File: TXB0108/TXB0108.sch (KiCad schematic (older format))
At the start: 6 parts, among them J1 Conn_01x10, J2 Conn_01x10, U1 TXB0108DQSR

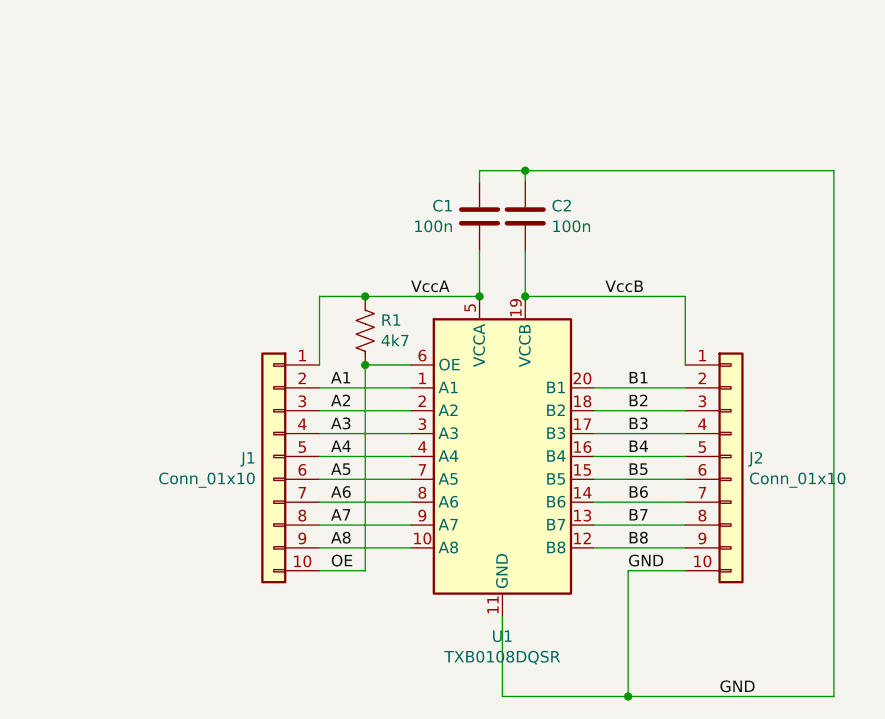
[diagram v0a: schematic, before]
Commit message: Part Numbers Added
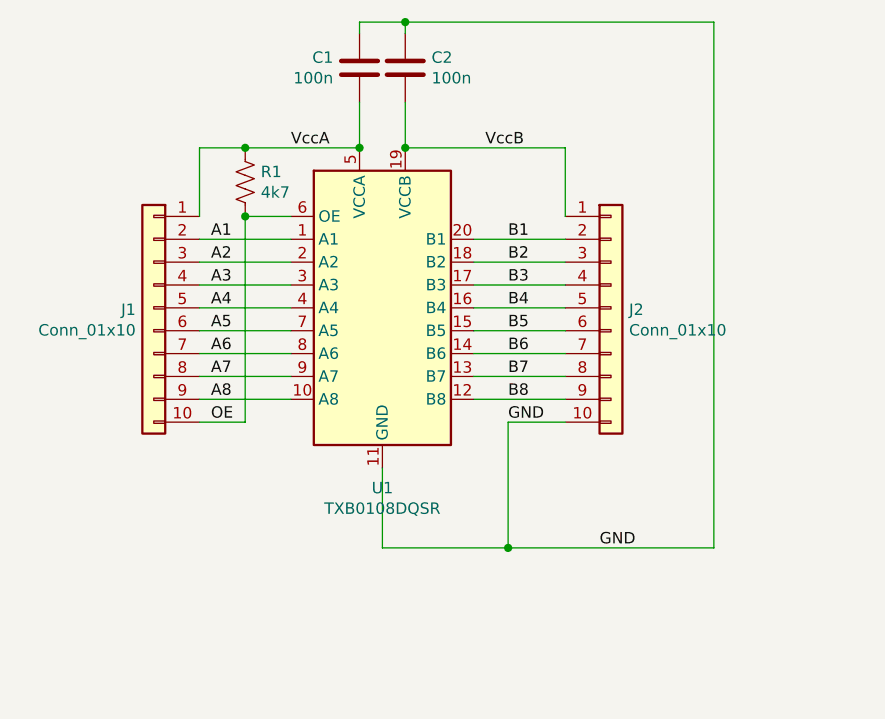
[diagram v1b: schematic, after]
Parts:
- C1, C2: Part (none) -> C38141
- R1: Part (none) -> C99782
- U1: Part (none) -> C53406
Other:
- moved on the sheet: C1, C2, J1, J2, R1, U1
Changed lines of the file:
@@
 EESchema Schematic File Version 4
+LIBS:TXB0108-cache
 EELAYER 29 0
 EELAYER END
-$Descr A4 11693 8268
+$Descr User 8268 5807
 encoding utf-8
 Sheet 1 1
-Title ""
-Date ""
-Rev ""
-Comp ""
-Comment1 ""
-Comment2 ""
-Comment3 ""
+Title "8 Channel Bi-Directional Level Shifter"
+Date "2019-09-16"
+Rev "1"
+Comp "SirBoard"
+Comment1 "www.SirBoard.com"
+Comment2 "TXB0108"
+Comment3 "SirLevel"
 Comment4 ""
 $EndDescr
@@
 L Logic_LevelTranslator:TXB0108DQSR U1
 U 1 1 5D2EEB39
-P 4250 3150
-F 0 "U1" H 4250 2362 50  0000 C CNN
-F 1 "TXB0108DQSR" H 4250 2272 50  0000 C CNN
-F 2 "Package_SO:TSSOP-20_4.4x6.5mm_P0.65mm" H 4250 2400 50  0001 C CNN
-F 3 "http://www.ti.com/lit/ds/symlink/txb0108.pdf" H 4250 3050 50  0001 C CNN
-	1    4250 3150
+P 3725 2500
+F 0 "U1" H 3725 1712 50  0000 C CNN
+F 1 "TXB0108DQSR" H 3725 1622 50  0000 C CNN
+F 2 "Package_SO:TSSOP-20_4.4x6.5mm_P0.65mm" H 3725 1750 50  0001 C CNN
+F 3 "http://www.ti.com/lit/ds/symlink/txb0108.pdf" H 3725 2400 50  0001 C CNN
+F 4 "C53406" H 3725 2500 50  0001 C CNN "Part"
+	1    3725 2500
 	1    0    0    -1
 $EndComp
@@
 L Connector_Generic:Conn_01x10 J2
 U 1 1 5D2EF020
-P 5250 3150
-F 0 "J2" H 5329 3142 50  0000 L CNN
-F 1 "Conn_01x10" H 5329 3052 50  0000 L CNN
-F 2 "Connector_PinHeader_2.54mm:PinHeader_1x10_P2.54mm_Vertical" H 5250 3150 50  0001 C CNN
-F 3 "~" H 5250 3150 50  0001 C CNN
-	1    5250 3150
+P 4725 2500
+F 0 "J2" H 4804 2492 50  0000 L CNN
+F 1 "Conn_01x10" H 4804 2402 50  0000 L CNN
+F 2 "Connector_PinHeader_2.54mm:PinHeader_1x10_P2.54mm_Vertical" H 4725 2500 50  0001 C CNN
+F 3 "~" H 4725 2500 50  0001 C CNN
+	1    4725 2500
 	1    0    0    -1
 $EndComp
@@
 L Connector_Generic:Conn_01x10 J1
 U 1 1 5D2F0A7B
-P 3250 3150
-F 0 "J1" H 3329 3142 50  0000 L CNN
-F 1 "Conn_01x10" H 3329 3052 50  0000 L CNN
-F 2 "Connector_PinHeader_2.54mm:PinHeader_1x10_P2.54mm_Vertical" H 3250 3150 50  0001 C CNN
-F 3 "~" H 3250 3150 50  0001 C CNN
-	1    3250 3150
+P 2725 2500
+F 0 "J1" H 2804 2492 50  0000 L CNN
+F 1 "Conn_01x10" H 2804 2402 50  0000 L CNN
+F 2 "Connector_PinHeader_2.54mm:PinHeader_1x10_P2.54mm_Vertical" H 2725 2500 50  0001 C CNN
+F 3 "~" H 2725 2500 50  0001 C CNN
+	1    2725 2500
 	-1   0    0    -1
 $EndComp
 Wire Wire Line
-	3850 2850 3450 2850
-Wire Wire Line
-	3850 2950 3450 2950
-Wire Wire Line
-	3850 3050 3450 3050
-Wire Wire Line
-	3850 3150 3450 3150
-Wire Wire Line
-	3850 3250 3450 3250
-Wire Wire Line
-	3850 3350 3450 3350
-Wire Wire Line
-	3850 3450 3450 3450
-Wire Wire Line
-	3850 3550 3450 3550
-Wire Wire Line
-	5050 2850 4650 2850
-Wire Wire Line
-	5050 2950 4650 2950
-Wire Wire Line
-	5050 3050 4650 3050
-Wire Wire Line
-	5050 3150 4650 3150
-Wire Wire Line
-	5050 3250 4650 3250
-Wire Wire Line
-	5050 3350 4650 3350
-Wire Wire Line
-	5050 3450 4650 3450
-Wire Wire Line
-	5050 3550 4650 3550
+	3325 2200 2925 2200
+Wire Wire Line
+	3325 2300 2925 2300
+Wire Wire Line
+	3325 2400 2925 2400
+Wire Wire Line
+	3325 2500 2925 2500
+Wire Wire Line
+	3325 2600 2925 2600
+Wire Wire Line
+	3325 2700 2925 2700
+Wire Wire Line
+	3325 2800 2925 2800
+Wire Wire Line
+	3325 2900 2925 2900
+Wire Wire Line
+	4525 2200 4125 2200
+Wire Wire Line
+	4525 2300 4125 2300
+Wire Wire Line
+	4525 2400 4125 2400
+Wire Wire Line
+	4525 2500 4125 2500
+Wire Wire Line
+	4525 2600 4125 2600
+Wire Wire Line
+	4525 2700 4125 2700
+Wire Wire Line
+	4525 2800 4125 2800
+Wire Wire Line
+	4525 2900 4125 2900
 $Comp
 L Device:C C1
 U 1 1 5D2F4CB8
-P 4150 2100
-F 0 "C1" H 4265 2145 50  0000 L CNN
-F 1 "100n" H 4265 2055 50  0000 L CNN
-F 2 "Capacitor_SMD:C_0805_2012Metric_Pad1.15x1.40mm_HandSolder" H 4188 1950 50  0001 C CNN
-F 3 "~" H 4150 2100 50  0001 C CNN
-	1    4150 2100
+P 3625 1450
+F 0 "C1" H 3740 1495 50  0000 L CNN
+F 1 "100n" H 3740 1405 50  0000 L CNN
+F 2 "Capacitor_SMD:C_0805_2012Metric_Pad1.15x1.40mm_HandSolder" H 3663 1300 50  0001 C CNN
+F 3 "~" H 3625 1450 50  0001 C CNN
+F 4 "C38141" H 3625 1450 50  0001 C CNN "Part"
+	1    3625 1450
 	-1   0    0    -1
 $EndComp
@@
 L Device:C C2
 U 1 1 5D2F688A
-P 4350 2100
-F 0 "C2" H 4235 2145 50  0000 R CNN
-F 1 "100n" H 4235 2055 50  0000 R CNN
-F 2 "Capacitor_SMD:C_0805_2012Metric_Pad1.15x1.40mm_HandSolder" H 4388 1950 50  0001 C CNN
-F 3 "~" H 4350 2100 50  0001 C CNN
-	1    4350 2100
+P 3825 1450
+F 0 "C2" H 3710 1495 50  0000 R CNN
+F 1 "100n" H 3710 1405 50  0000 R CNN
+F 2 "Capacitor_SMD:C_0805_2012Metric_Pad1.15x1.40mm_HandSolder" H 3863 1300 50  0001 C CNN
+F 3 "~" H 3825 1450 50  0001 C CNN
+F 4 "C38141" H 3825 1450 50  0001 C CNN "Part"
+	1    3825 1450
 	-1   0    0    -1
 $EndComp
 Wire Wire Line
-	4150 2450 4150 2250
-Wire Wire Line
-	4350 1900 4150 1900
-Wire Wire Line
-	4150 1900 4150 1950
-Wire Wire Line
-	4350 1950 4350 1900
-Wire Wire Line
-	4350 2250 4350 2450
-Wire Wire Line
-	4250 3850 4250 4200
-Wire Wire Line
-	4250 4200 4800 4200
-Wire Wire Line
-	5700 4200 5700 1900
-Wire Wire Line
-	5700 1900 4350 1900
-Connection ~ 4350 1900
-Wire Wire Line
-	3450 2750 3450 2450
-Wire Wire Line
-	3450 2450 3650 2450
-Connection ~ 4150 2450
-Wire Wire Line
-	4350 2450 5050 2450
-Wire Wire Line
-	5050 2450 5050 2750
-Connection ~ 4350 2450
-Wire Wire Line
-	3850 2750 3650 2750
-Wire Wire Line
-	3650 2750 3650 3650
-Wire Wire Line
-	3650 3650 3450 3650
+	3625 1800 3625 1600
+Wire Wire Line
+	3825 1250 3625 1250
+Wire Wire Line
+	3625 1250 3625 1300
+Wire Wire Line
+	3825 1300 3825 1250
+Wire Wire Line
+	3825 1600 3825 1800
+Wire Wire Line
+	3725 3200 3725 3550
+Wire Wire Line
+	3725 3550 4275 3550
+Wire Wire Line
+	5175 3550 5175 1250
+Wire Wire Line
+	5175 1250 3825 1250
+Connection ~ 3825 1250
+Wire Wire Line
+	2925 2100 2925 1800
+Wire Wire Line
+	2925 1800 3125 1800
+Connection ~ 3625 1800
+Wire Wire Line
+	3825 1800 4525 1800
+Wire Wire Line
+	4525 1800 4525 2100
+Connection ~ 3825 1800
+Wire Wire Line
+	3325 2100 3125 2100
+Wire Wire Line
+	3125 2100 3125 3000
+Wire Wire Line
+	3125 3000 2925 3000
 $Comp
 L Device:R_US R1
 U 1 1 5D2FDFC2
-P 3650 2600
-F 0 "R1" H 3718 2645 50  0000 L CNN
-F 1 "4k7" H 3718 2555 50  0000 L CNN
-F 2 "Resistor_SMD:R_0805_2012Metric_Pad1.15x1.40mm_HandSolder" V 3690 2590 50  0001 C CNN
-F 3 "~" H 3650 2600 50  0001 C CNN
-	1    3650 2600
+P 3125 1950
+F 0 "R1" H 3193 1995 50  0000 L CNN
+F 1 "4k7" H 3193 1905 50  0000 L CNN
+F 2 "Resistor_SMD:R_0805_2012Metric_Pad1.15x1.40mm_HandSolder" V 3165 1940 50  0001 C CNN
+F 3 "~" H 3125 1950 50  0001 C CNN
+F 4 "C99782" H 3125 1950 50  0001 C CNN "Part"
+	1    3125 1950
 	1    0    0    -1
 $EndComp
-Connection ~ 3650 2450
-Wire Wire Line
-	3650 2450 4150 2450
-Connection ~ 3650 2750
-Wire Wire Line
-	5050 3650 4800 3650
-Wire Wire Line
-	4800 3650 4800 4200
-Connection ~ 4800 4200
-Wire Wire Line
-	4800 4200 5700 4200
-Text Label 4700 2450 0    50   ~ 0
+Connection ~ 3125 1800
+Wire Wire Line
+	3125 1800 3625 1800
+Connection ~ 3125 2100
+Wire Wire Line
+	4525 3000 4275 3000
+Wire Wire Line
+	4275 3000 4275 3550
+Connection ~ 4275 3550
+Wire Wire Line
+	4275 3550 5175 3550
+Text Label 4175 1800 0    50   ~ 0
 VccB
-Text Label 3850 2450 0    50   ~ 0
+Text Label 3325 1800 0    50   ~ 0
 VccA
-Text Label 3500 2850 0    50   ~ 0
+Text Label 2975 2200 0    50   ~ 0
 A1
-Text Label 3500 2950 0    50   ~ 0
+Text Label 2975 2300 0    50   ~ 0
 A2
-Text Label 3500 3050 0    50   ~ 0
+Text Label 2975 2400 0    50   ~ 0
 A3
-Text Label 3500 3150 0    50   ~ 0
+Text Label 2975 2500 0    50   ~ 0
 A4
-Text Label 3500 3250 0    50   ~ 0
+Text Label 2975 2600 0    50   ~ 0
 A5
-Text Label 3500 3350 0    50   ~ 0
+Text Label 2975 2700 0    50   ~ 0
 A6
-Text Label 3500 3450 0    50   ~ 0
+Text Label 2975 2800 0    50   ~ 0
 A7
-Text Label 3500 3550 0    50   ~ 0
+Text Label 2975 2900 0    50   ~ 0
 A8
-Text Label 3500 3650 0    50   ~ 0
+Text Label 2975 3000 0    50   ~ 0
 OE
-Text Label 4800 3550 0    50   ~ 0
+Text Label 4275 2900 0    50   ~ 0
 B8
-Text Label 4800 3650 0    50   ~ 0
+Text Label 4275 3000 0    50   ~ 0
 GND
-Text Label 4800 3450 0    50   ~ 0
+Text Label 4275 2800 0    50   ~ 0
 B7
-Text Label 4800 3350 0    50   ~ 0
+Text Label 4275 2700 0    50   ~ 0
 B6
-Text Label 4800 3250 0    50   ~ 0
+Text Label 4275 2600 0    50   ~ 0
 B5
-Text Label 4800 3150 0    50   ~ 0
+Text Label 4275 2500 0    50   ~ 0
 B4
-Text Label 4800 3050 0    50   ~ 0
+Text Label 4275 2400 0    50   ~ 0
 B3
-Text Label 4800 2950 0    50   ~ 0
+Text Label 4275 2300 0    50   ~ 0
 B2
-Text Label 4800 2850 0    50   ~ 0
+Text Label 4275 2200 0    50   ~ 0
 B1
-Text Label 5200 4200 0    50   ~ 0
+Text Label 4675 3550 0    50   ~ 0
 GND
 $EndSCHEMATC
